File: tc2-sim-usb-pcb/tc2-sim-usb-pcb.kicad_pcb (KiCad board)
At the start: 4 copper layers, 19.5 x 56 mm, 9 parts, among them J2 Conn_01x08

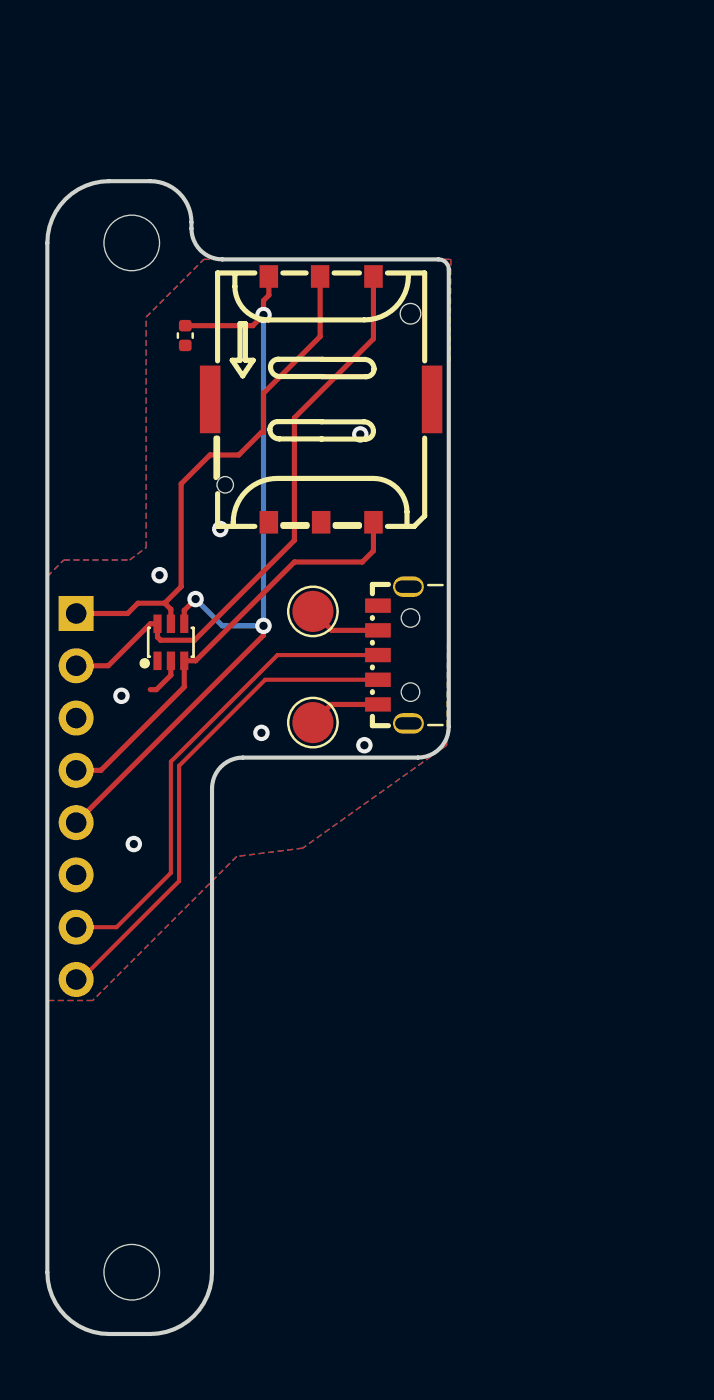
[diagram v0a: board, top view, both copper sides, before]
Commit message: P3-Nov release
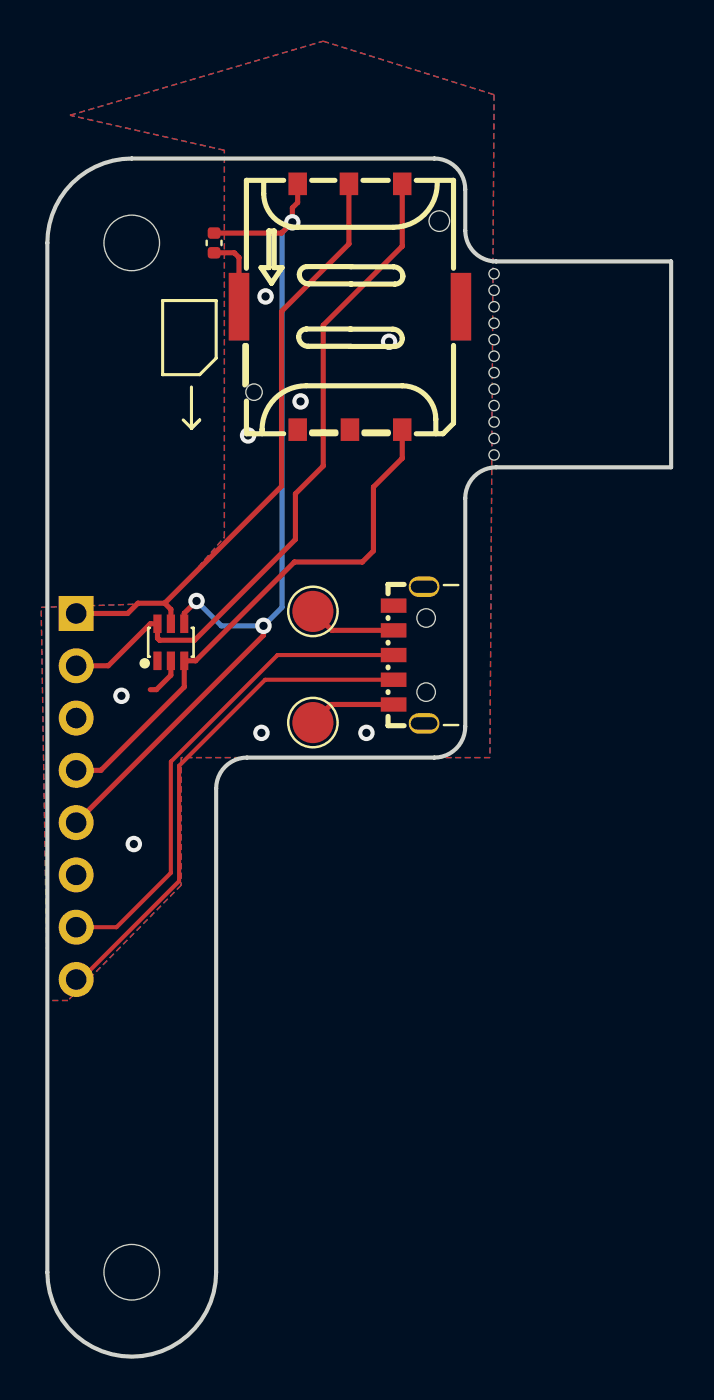
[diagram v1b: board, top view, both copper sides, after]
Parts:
- added H3: MountingHole, cacophony-library:mouse-bite-10mm, F.Cu at (20.3, -7.10)
- H1, H2: footprint MountingHole:MountingHole_2.7mm_M2.5 -> cacophony-library:MountingHole_2.7mm_M2.5
- moved C2 4.71 mm to (6.70, -18.0)
- moved Card1 4.71 mm to (13.3, -14.9)
- moved USB2 0.76 mm to (16.2, 2.02)
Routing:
- net USIM_CLK: track 28.6 -> 33.7 mm
- net USIM_DATA: track 21.0 -> 26.1 mm
- net USIM_VDD: track 39.7 -> 44.6 mm
- net USIM_RST: track 25.5 -> 29.7 mm
- net GND: track 1.99 -> 5.69 mm, vias 7 -> 8
- net 4G_USB_D-: track 24.0 -> 24.7 mm
- net Net-(USB2-ID): track 3.54 -> 4.30 mm
- net Net-(USB2-VBUS): track 3.52 -> 4.28 mm
- net 4G_USB_D+: track 23.3 -> 24.1 mm
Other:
- board size 19.5 x 56 mm -> 30.3 x 58.2 mm
